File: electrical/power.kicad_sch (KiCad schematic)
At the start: 5 parts

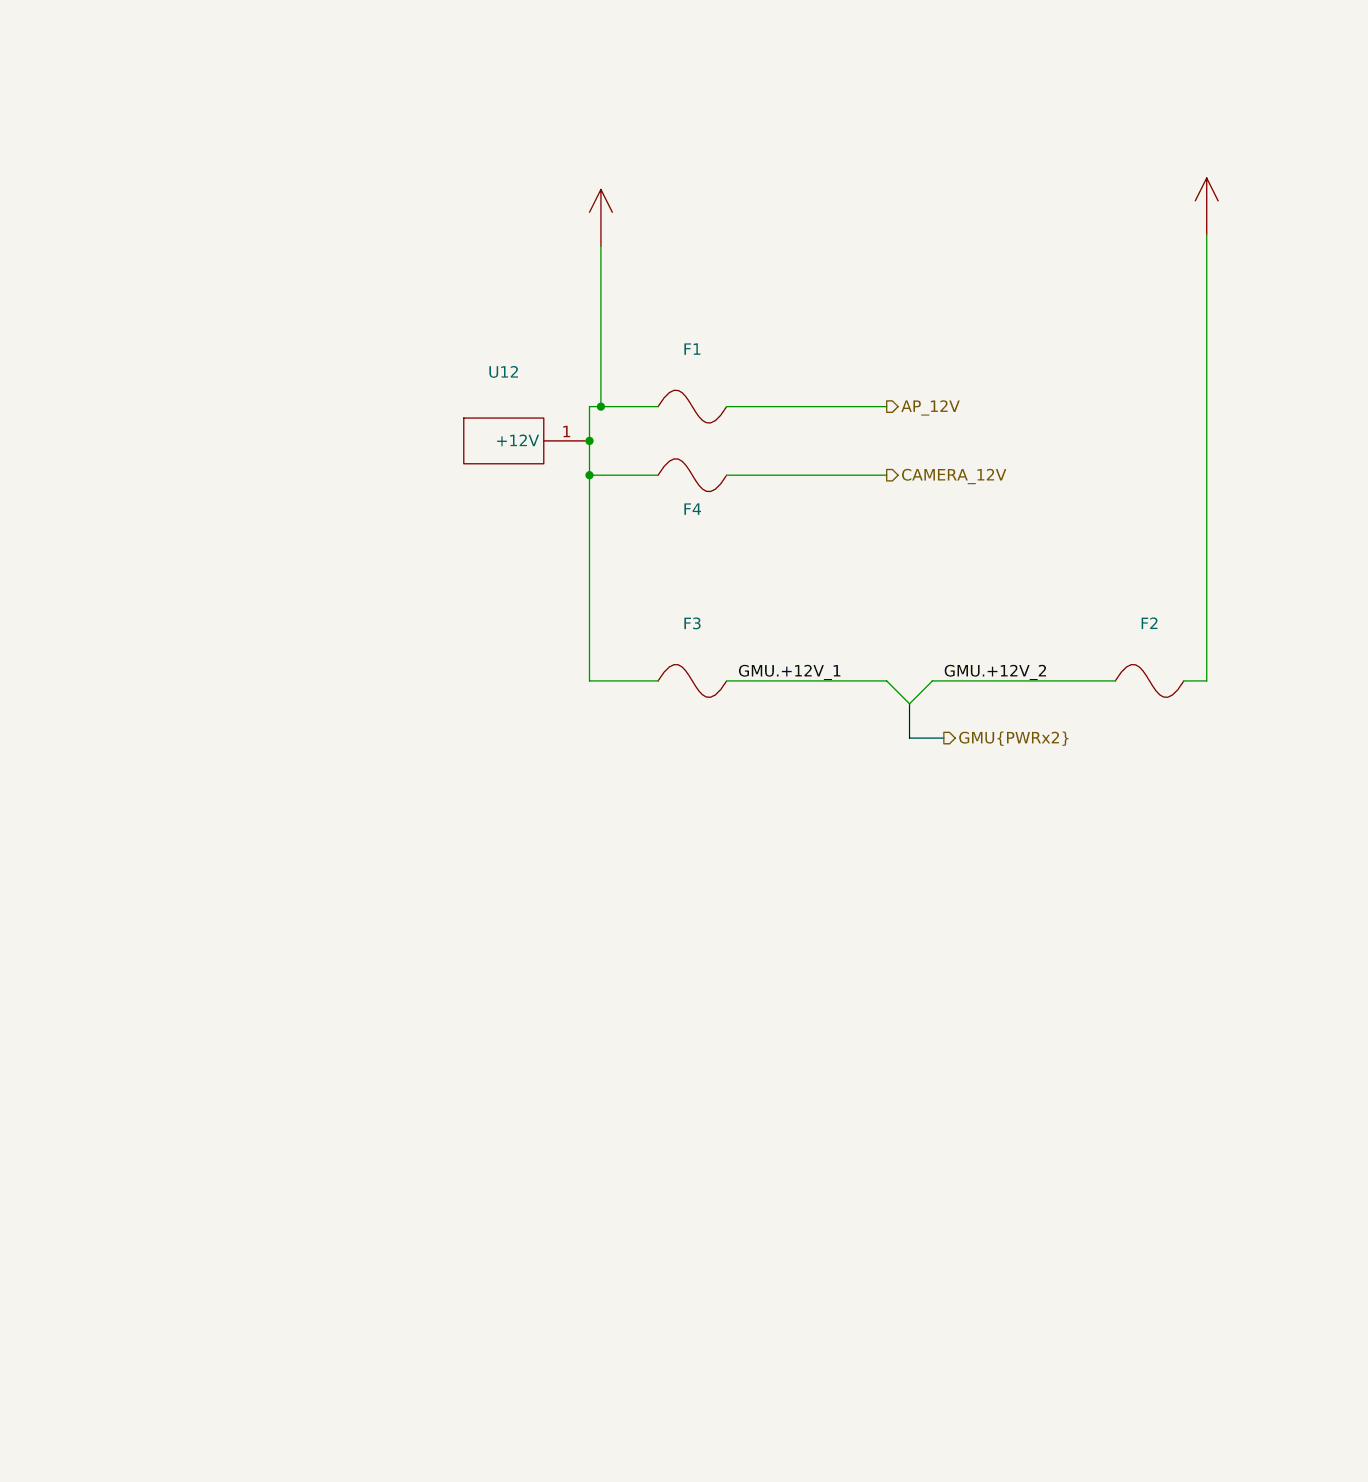
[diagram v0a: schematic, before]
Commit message: 🎮 Working on electrical schematic
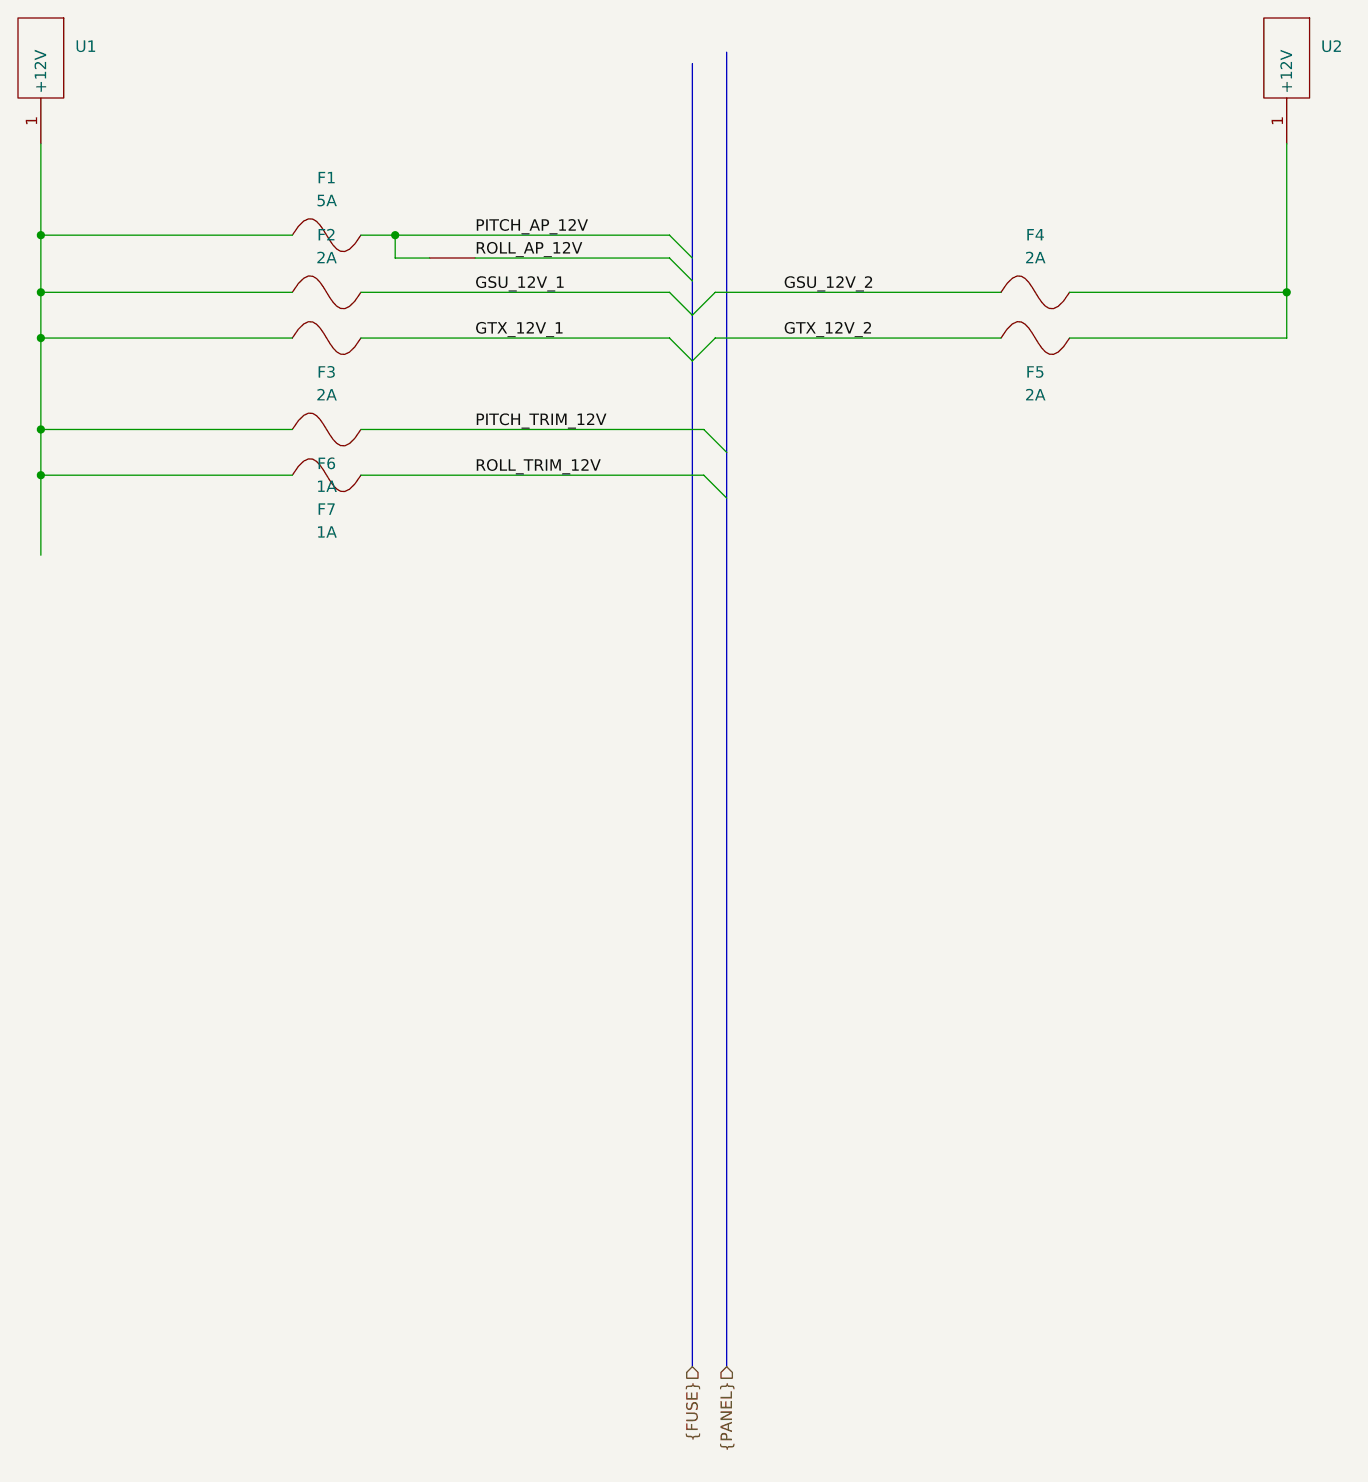
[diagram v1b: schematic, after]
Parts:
- removed U12: ~, symbol Misc:BAT
- added F5: 2A, symbol Misc:FUSE
- added F6, F7: 1A, symbol Misc:FUSE
- added U1, U2: ~, symbol Misc:BAT
- added U3: ~, symbol Misc:TIE
- F1: value ~ -> 5A
- F2, F3, F4: value ~ -> 2A
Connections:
- net 12V: no longer names the net of F1.1, F2.1, F3.1
- net 12V: now also F6.1, F7.1, U1.1 (+12V); no longer F4.1
- net AP_12V renamed PITCH_AP_12V
- net PITCH_AP_12V: now also U3.1
- net CAMERA_12V renamed GSU_12V_2
- net GMU.+12V_1 renamed GTX_12V_1
- net GMU.+12V_2 renamed GSU_12V_1
- new net: F4.1, F5.1, U2.1 (+12V)
- new net GTX_12V_2: F5.2
- new net PITCH_TRIM_12V: F6.2
- new net ROLL_AP_12V: U3.2
- new net ROLL_TRIM_12V: F7.2
